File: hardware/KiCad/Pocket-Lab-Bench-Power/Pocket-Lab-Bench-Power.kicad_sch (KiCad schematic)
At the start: 157 parts, among them J1 Conn_01x05_Pin, J2 Conn_01x04_Pin, J3 Conn_01x04_Pin, J4 Conn_01x02, Q1 CSD87501L, SW1 PS-5850A-6PL, U1 TVS2200DRV, U11 DC-S011A-D025-20A, U12 TPS259474ARPWR, U13 STM32L031G6Ux, U15 SY8253ADC, U2 TPS25730SRSMR, U3 BQ25792RQMR, U4 INA226, U5 SY8253ADC, U6 TPS55289RYQR, U7 INA226, U8 ESD122DMYR, U9 TPS70933DBVR

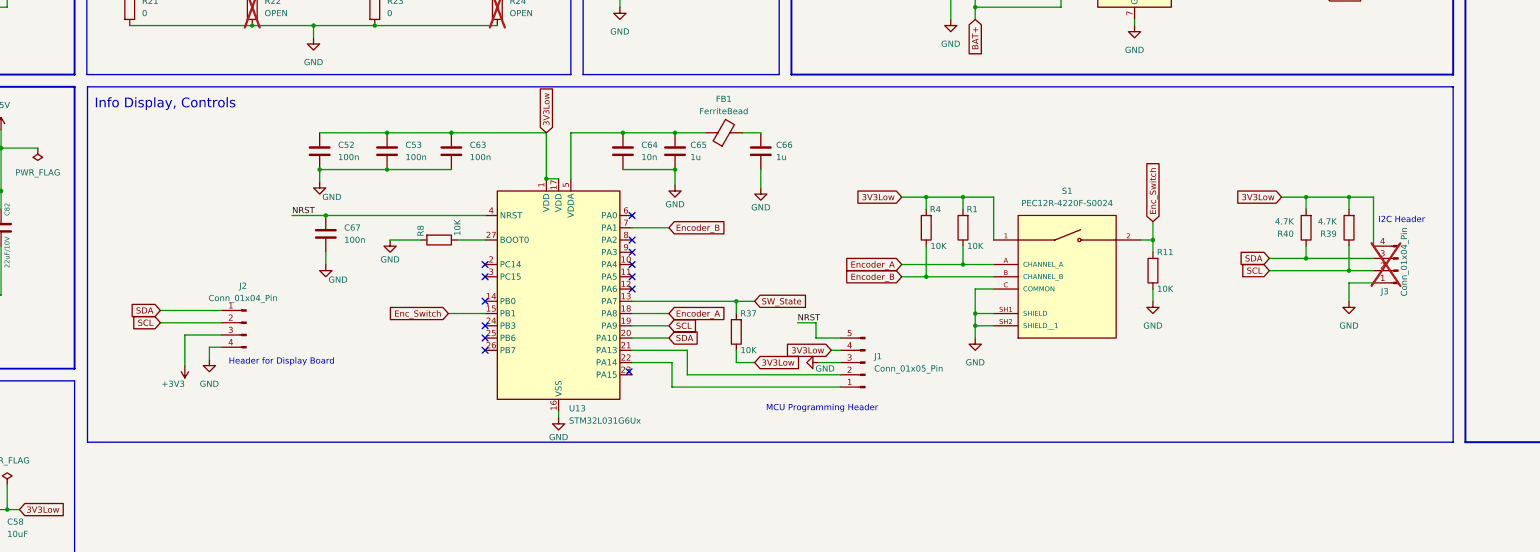
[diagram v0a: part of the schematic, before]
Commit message: PCB routing #1
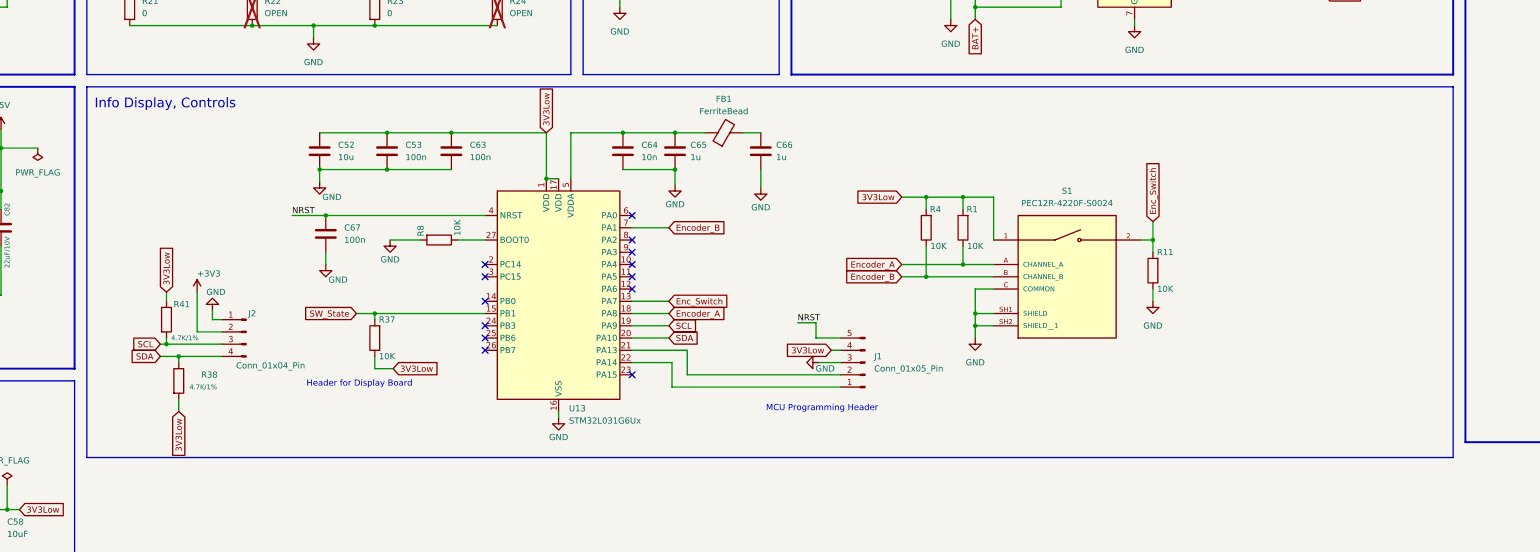
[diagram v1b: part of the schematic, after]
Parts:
- removed J3: Conn_01x04_Pin, Connector_PinHeader_2.54mm:PinHeader_1x04_P2.54mm_Vertical, symbol Connector:Conn_01x04_Pin
- removed R39, R40: 4.7K, Resistor_SMD:R_0603_1608Metric, symbol Device:R
- added R38, R41: 4.7K/1%, Resistor_SMD:R_0603_1608Metric, symbol Device:R
- C52: value 100n -> 10u; footprint Capacitor_SMD:C_0201_0603Metric -> Capacitor_SMD:C_0603_1608Metric; LCSC C7393837 -> C19702
- C53, C63, C67: footprint Capacitor_SMD:C_0201_0603Metric -> Capacitor_SMD:C_0402_1005Metric; LCSC C7393837 -> C1525
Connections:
- net +3V3: now also J2.2 (Pin_2); no longer J2.3 (Pin_3)
- net 3V3Low: now also R38.2, R41.1
- net Enc_Switch: now also U13.13 (PA7); no longer U13.15 (PB1)
- net GND: now also J2.1 (Pin_1); no longer J2.4 (Pin_4)
- net SCL: now also J2.3 (Pin_3), R41.2; no longer J2.2 (Pin_2)
- net SDA: now also J2.4 (Pin_4), R38.1; no longer J2.1 (Pin_1)
- net SW_State: now also U13.15 (PB1); no longer U13.13 (PA7)
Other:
- note removed: "I2C Header"
- moved on the sheet: J2, R37
